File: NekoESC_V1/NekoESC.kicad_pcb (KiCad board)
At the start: 4 copper layers, 38.5 x 38.5 mm, 174 parts, among them J101 SWD, J102 SWD, J107 JST-SH_8P, Q201 NMOS, Q202 NMOS, Q203 NMOS, Q204 NMOS, Q205 NMOS, Q206 NMOS, Q301 NMOS, Q302 NMOS, Q303 NMOS, Q304 NMOS, Q305 NMOS, Q306 NMOS, Q401 NMOS, Q402 NMOS, Q403 NMOS, Q404 NMOS, Q405 NMOS, Q406 NMOS, Q501 NMOS, Q502 NMOS, Q503 NMOS, Q504 NMOS, Q505 NMOS, Q506 NMOS, U102 ME3121, U103 INA180A1, U104 HT7533-1-SOT89, U201 GD32E230G8U6, U202 FD6288Q, U301 GD32E230G8U6, U302 FD6288Q, U401 GD32E230G8U6, U402 FD6288Q, U501 GD32E230G8U6, U502 FD6288Q

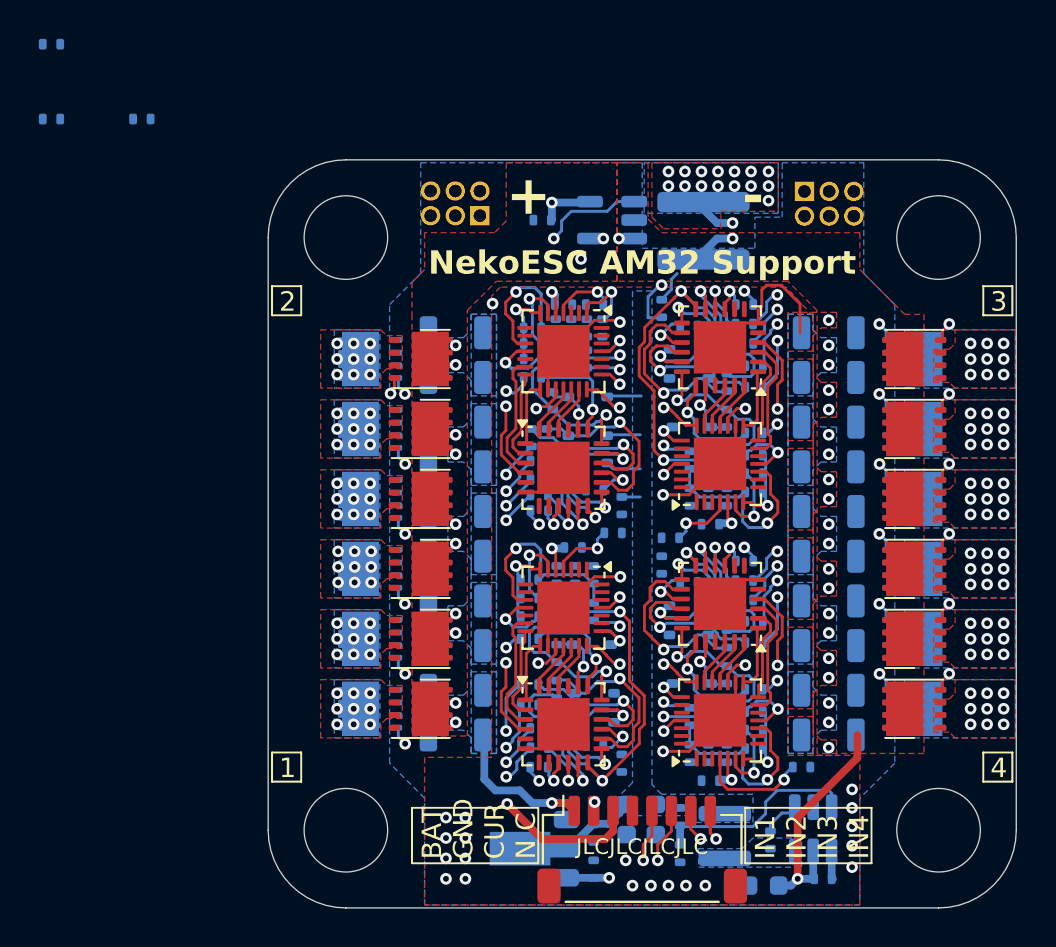
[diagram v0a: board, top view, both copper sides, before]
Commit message: update lib
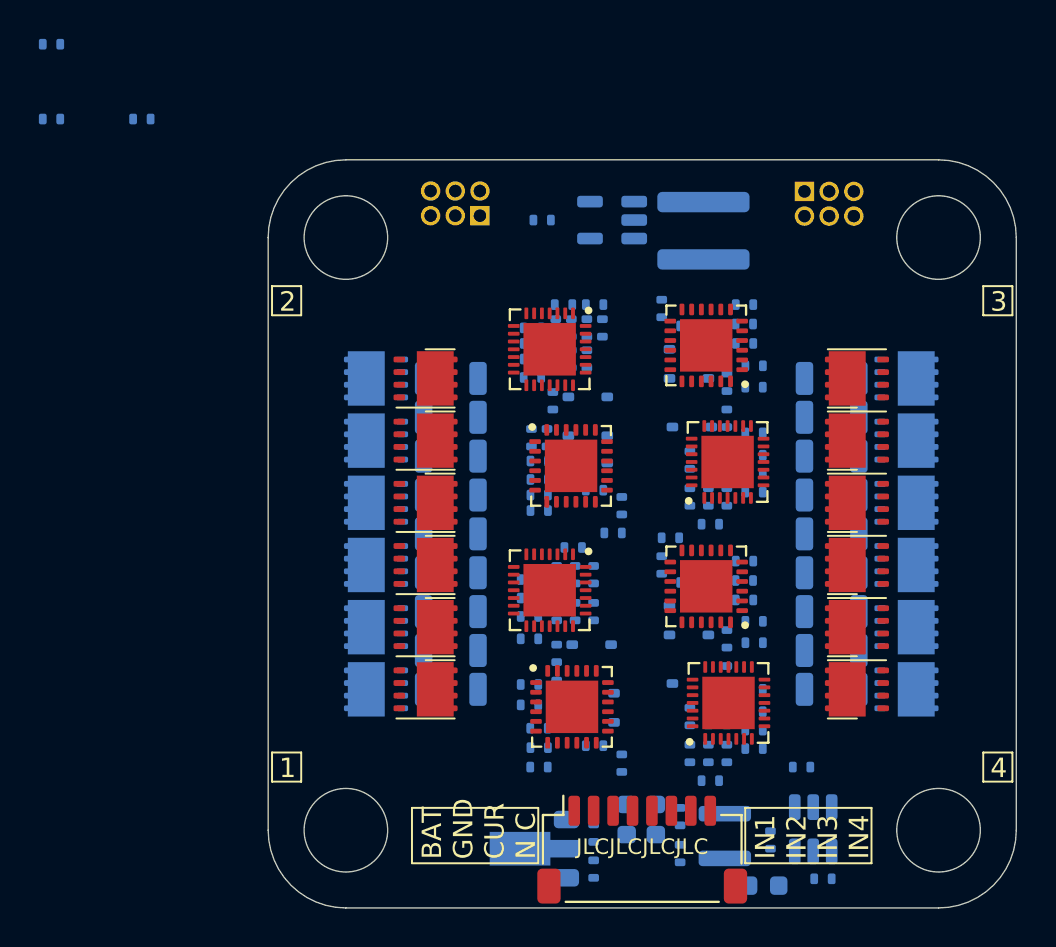
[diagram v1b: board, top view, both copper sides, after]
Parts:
- removed C147, C163: 10uF/50V, SMTOPT:C_1206
- U201, U301, U401, U501: footprint Package_DFN_QFN:WQFN-28-1EP_4x4mm_P0.4mm_EP2.7x2.7mm -> SMTOPT:WQFN-28-1EP_4x4mm_P0.4mm_EP2.7x2.7mm
- U202, U302, U402, U502: footprint Package_DFN_QFN:QFN-24-1EP_4x4mm_P0.5mm_EP2.7x2.7mm -> SMTOPT:QFN-24-1EP_4x4mm_P0.5mm_EP2.7x2.7mm
- moved Q503 3.11 mm to (126.0, 107.0)
- moved Q401 3.11 mm to (126.0, 123.0)
- moved Q502 3.01 mm to (126.0, 110.2)
- moved Q402 3.01 mm to (126.0, 119.8)
- moved Q501 2.96 mm to (126.0, 113.4)
- moved Q403 2.96 mm to (126.0, 116.6)
- moved C138 2.36 mm to (105.2, 123.0)
- moved C134 2.35 mm to (124.8, 123.0)
- moved C139 2.07 mm to (105.2, 121.0)
- moved C136 2.06 mm to (124.8, 121.0)
- moved C140 1.77 mm to (105.2, 119.0)
- moved C149 1.76 mm to (124.8, 119.0)
- moved C141 1.47 mm to (105.2, 117.0)
- moved C151 1.46 mm to (124.8, 117.0)
- moved C142 1.18 mm to (105.2, 115.0)
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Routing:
- net +3V3: track 89.1 -> 0.00 mm, vias 10 -> 0
- net VCC: track 78.4 -> 0.00 mm, vias 5 -> 0
- net GND: track 52.4 -> 0.00 mm, vias 37 -> 0
- net /ISNS: track 50.8 -> 0.00 mm, vias 3 -> 0
- net /ESC4/VS_C1: track 39.4 -> 0.00 mm, vias 11 -> 0
- net /ESC3/VS_C1: track 38.7 -> 0.00 mm, vias 11 -> 0
- net /SWDIO3: track 36.2 -> 0.00 mm, vias 1 -> 0
- net /SWCLK2: track 35.5 -> 0.00 mm, vias 1 -> 0
- net /SWCLK3: track 32.5 -> 0.00 mm, vias 1 -> 0
- net /DSHOT1: track 31.8 -> 0.00 mm, vias 2 -> 0
- net /ESC3/VS_B1: track 31.4 -> 0.00 mm, vias 11 -> 0
- net /ESC4/VS_B1: track 31.3 -> 0.00 mm, vias 11 -> 0
- net /ESC2/VS_C1: track 31.1 -> 0.00 mm, vias 11 -> 0
- net /SWDIO2: track 30.7 -> 0.00 mm, vias 1 -> 0
- net /ESC1/VS_C1: track 29.0 -> 0.00 mm, vias 11 -> 0
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- removed copper zone on B.Cu, net /ESC1/VS_A1
- removed copper zone on F.Cu, net /ESC1/VS_A1
- removed copper zone on B.Cu, net /ESC1/VS_B1
- removed copper zone on F.Cu, net /ESC1/VS_B1
- removed copper zone on B.Cu, net /ESC1/VS_C1
- removed copper zone on F.Cu, net /ESC1/VS_C1
- removed copper zone on B.Cu, net /ESC2/VS_A1
- removed copper zone on F.Cu, net /ESC2/VS_A1
- removed copper zone on B.Cu, net /ESC2/VS_B1
- removed copper zone on F.Cu, net /ESC2/VS_B1
- removed copper zone on B.Cu, net /ESC2/VS_C1
- removed copper zone on F.Cu, net /ESC2/VS_C1
- removed copper zone on B.Cu, net /ESC3/VS_A1
- removed copper zone on F.Cu, net /ESC3/VS_A1
- removed copper zone on B.Cu, net /ESC3/VS_B1
- removed copper zone on F.Cu, net /ESC3/VS_B1
- removed copper zone on B.Cu, net /ESC3/VS_C1
- removed copper zone on F.Cu, net /ESC3/VS_C1
- removed copper zone on B.Cu, net /ESC4/VS_A1
- removed copper zone on F.Cu, net /ESC4/VS_A1
- removed copper zone on B.Cu, net /ESC4/VS_B1
- removed copper zone on F.Cu, net /ESC4/VS_B1
- removed copper zone on B.Cu, net /ESC4/VS_C1
- removed copper zone on F.Cu, net /ESC4/VS_C1
- removed copper zone on B.Cu, net /LX1
- removed copper zone on B.Cu, net GND
- removed copper zone on F.Cu, net GND
- removed copper zone on In1.Cu, net GND
- removed copper zone on In2.Cu, net GND
- removed copper zone on B.Cu, net GNDPWR
- removed copper zone on F.Cu, net GNDPWR
- removed copper zone on B.Cu, net VBUS
- removed copper zone on F.Cu, net VBUS
- removed copper zone on B.Cu, net VCC
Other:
- board text removed: "+"
- board text removed: "-"
- board text removed: "2025/09/27"
- board text removed: "@DuckWang"
- board text removed: "HW Rev 1.0"
- board text removed: "NekoESC"
- board text removed: "NekoESC AM32 Support"
